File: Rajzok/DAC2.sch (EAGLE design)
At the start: 17 parts, among them Q1 TP0602N2, Q2 TP0602N2, Q3 SUP75N06-08, Q4 SUP75N06-08

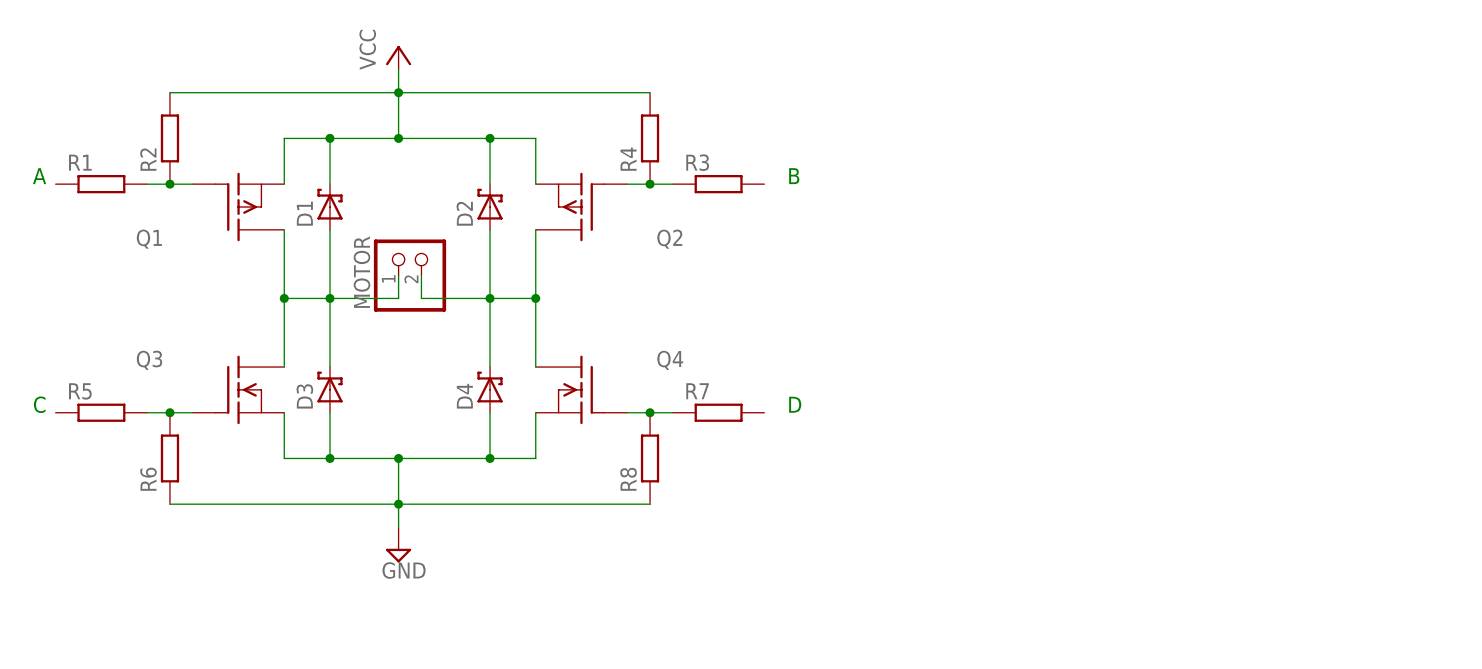
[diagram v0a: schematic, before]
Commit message: Rajzok 2017
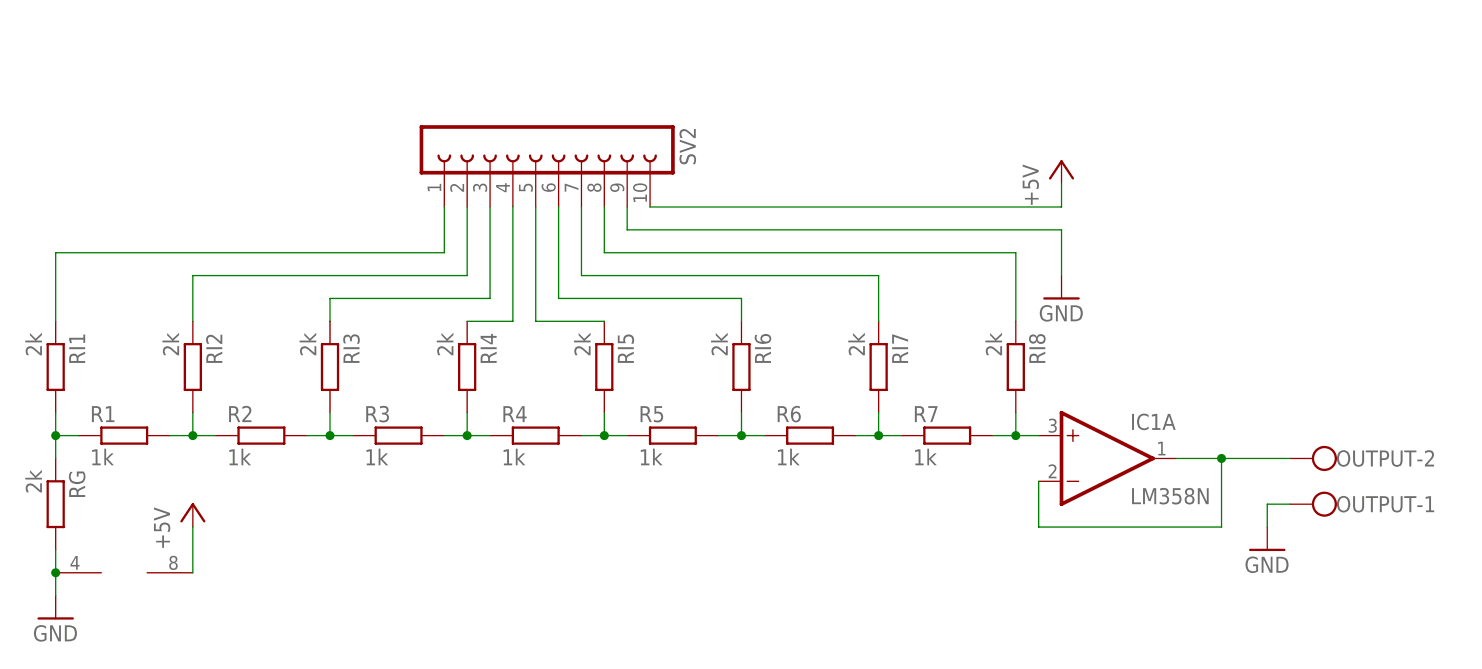
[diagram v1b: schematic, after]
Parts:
- removed D1, D2, D3, D4: 1N6267A, diode:1N6267A
- removed MOTOR: (no value), pinhead:PINHD-1X2
- removed Q1, Q2: TP0602N2, transistor-fet:TP0602N2
- removed Q3, Q4: SUP75N06-08, transistor-fet:SUP75N06-08
- removed R8: (no value), rcl:R-EU_0204/7
- added IC1: LM358N, linear:LM358N
- added OUTPUT: (no value), con-wago-500:W237-102
- added RG, RI1, RI2, RI3, RI4, RI5, RI6, RI7, RI8: 2k, rcl:R-EU_0207/12
- added SV2: (no value), con-lsta:FE10-1
- R1, R2, R3, R4, R5, R6, R7: value (none) -> 1k; device rcl:R-EU_0204/7 -> rcl:R-EU_0207/12
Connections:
- removed net VCC: D1.C, D2.C, Q1.S, Q2.S, R2.2, R4.2
- new net +5V: IC1P.V+, SV2.10
- new net N$10: RI1.1, SV2.1
- new net N$11: RI2.1, SV2.2
- new net N$12: RI3.1, SV2.3
- new net N$13: RI4.1, SV2.4
- new net N$14: RI5.1, SV2.5
- new net N$15: RI6.1, SV2.6
- new net N$16: RI7.1, SV2.7
- new net N$17: RI8.1, SV2.8
- new net N$6: R5.2, R6.1, RI6.2
- new net N$7: R6.2, R7.1, RI7.2
- new net N$8: IC1A.+IN, R7.2, RI8.2
- net GND: now also IC1P.V-, OUTPUT-1.KL, RG.2, SV2.9; no longer D3.A, D4.A, Q3.S, Q4.S, R6.1, R8.1
- net N$1: now also R1.1, RG.1, RI1.2; no longer Q1.G, R1.2, R2.1
- net N$2: now also R1.2, R2.1, RI2.2; no longer D2.A, D4.C, MOTOR.2, Q2.D, Q4.D
- net N$3: now also R2.2, RI3.2; no longer Q2.G, R4.1
- net N$4: now also R3.2, R4.1, RI4.2; no longer Q3.G, R5.2, R6.2
- net N$5: now also R4.2, R5.1, RI5.2; no longer Q4.G, R7.1, R8.2
- net N$9: now also IC1A.-IN, IC1A.OUT, OUTPUT-2.KL; no longer D1.A, D3.C, MOTOR.1, Q1.D, Q3.D
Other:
- note removed: "A"
- note removed: "B"
- note removed: "C"
- note removed: "D"
- moved on the sheet: R1, R2, R3, R4, R5, R6, R7
